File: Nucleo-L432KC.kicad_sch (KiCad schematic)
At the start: 8 parts, among them U1 Nucleo_L432KC

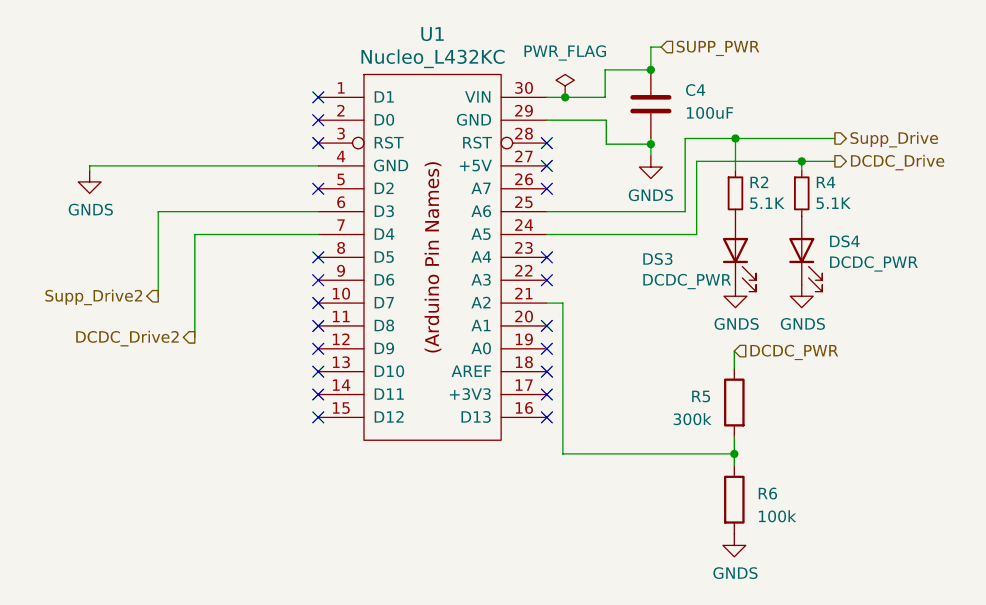
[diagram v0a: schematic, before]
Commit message: Schematic redesign
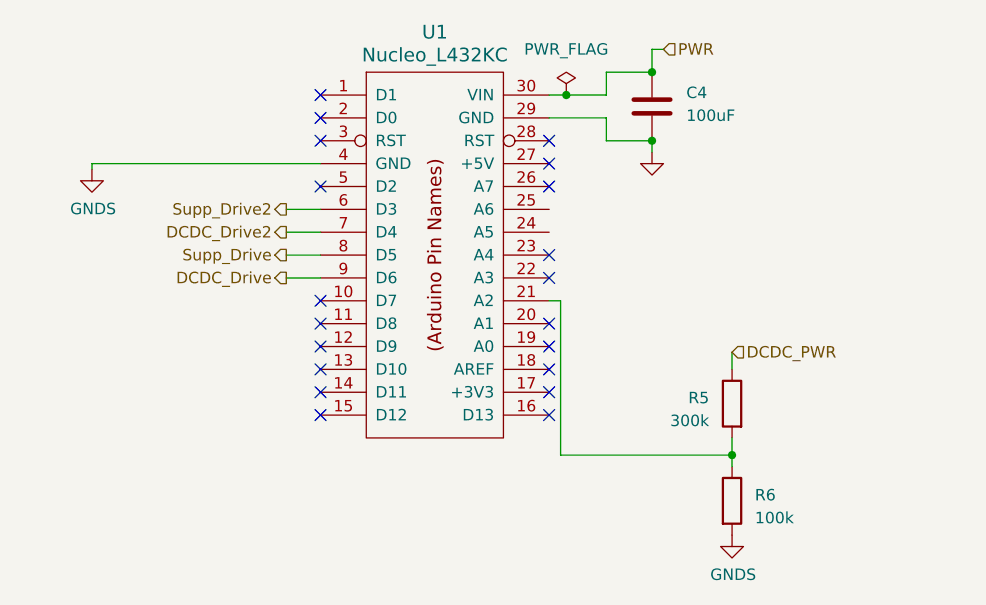
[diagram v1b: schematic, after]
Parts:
- removed DS3, DS4: DCDC_PWR, Diode_SMD:D_0805_2012Metric, symbol Device:LED
- removed R2, R4: 5.1K, Resistor_SMD:R_0805_2012Metric, symbol Device:R_Small
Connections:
- net DCDC_Drive: now also U1.9 (D6); no longer U1.24 (A5)
- net Supp_Drive: now also U1.8 (D5); no longer U1.25 (A6)
- net SUPP_PWR renamed PWR
- no-connect marks 22 -> 20
